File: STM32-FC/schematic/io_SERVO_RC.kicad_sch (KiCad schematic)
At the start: 10 parts, among them J5 PWM_Conn_3x04, J6 PWM_Conn_3x04, J7 PWM_Conn_3x04, J8 ZH 1.5mm 4P, J9 GH 1.25mm 4P, Q1 PMDPB30XN

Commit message: WIP : pcb part layout &* BOM udpate
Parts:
- J5, J6, J7: LCSC C3327492 -> C3325573
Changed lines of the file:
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@@
 			)
 		)
-		(property "LCSC" "C3327492"
+		(property "LCSC" "C3325573"
 			(at 120.65 58.42 0)
 			(effects
@@
 			)
 		)
-		(property "LCSC" "C3327492"
+		(property "LCSC" "C3325573"
 			(at 55.88 52.07 0)
 			(effects
@@
 			)
 		)
-		(property "LCSC" "C3327492"
+		(property "LCSC" "C3325573"
 			(at 55.88 74.93 0)
 			(effects

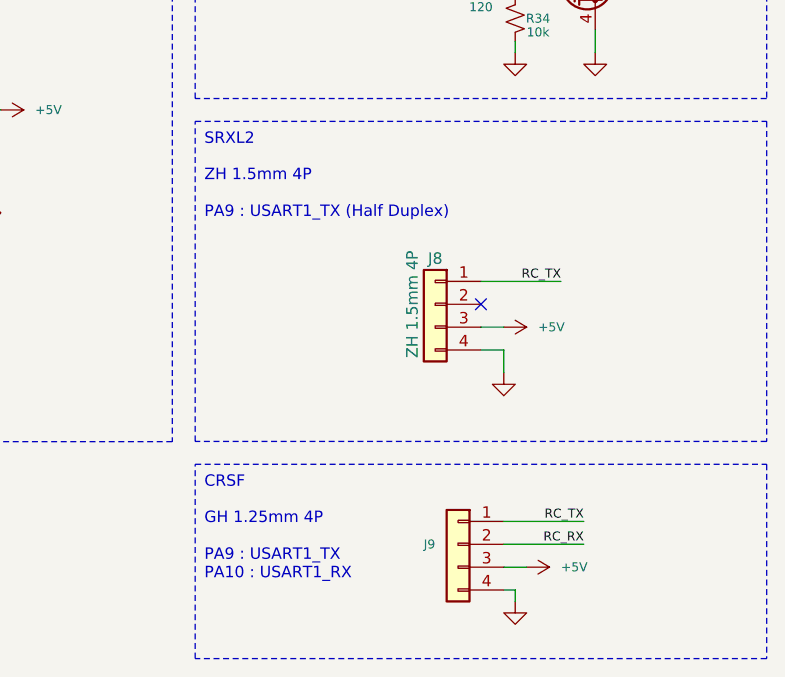
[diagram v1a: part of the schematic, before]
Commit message: update : AHRS PCB layout & routing done
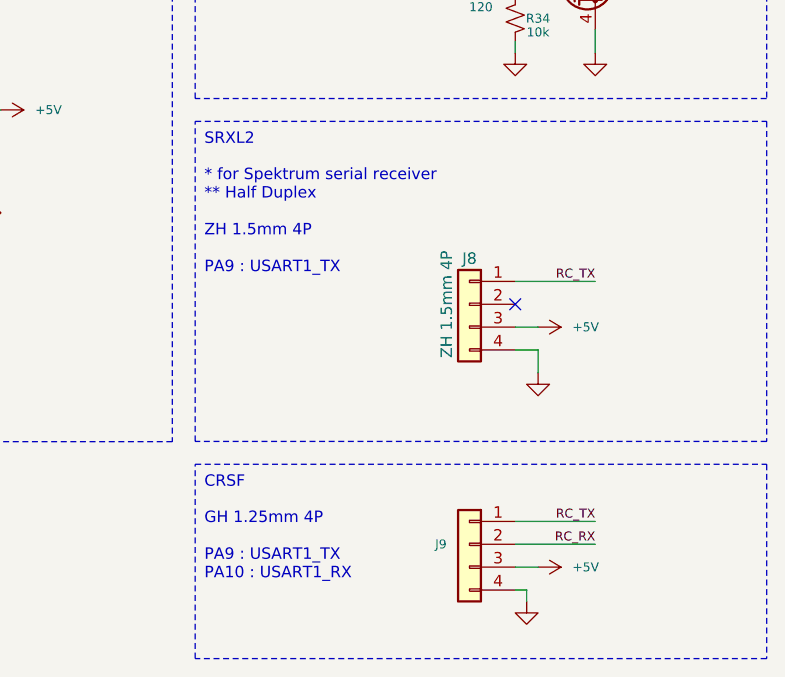
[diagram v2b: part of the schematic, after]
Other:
- note added: "* for Spektrum serial receiver ** Half Duplex ZH 1.5mm 4P PA9 : USART1_TX"
- note removed: "ZH 1.5mm 4P PA9 : USART1_TX (Half Duplex)"
- moved on the sheet: J8, J9
